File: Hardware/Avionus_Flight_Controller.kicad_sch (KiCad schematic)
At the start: 0 parts

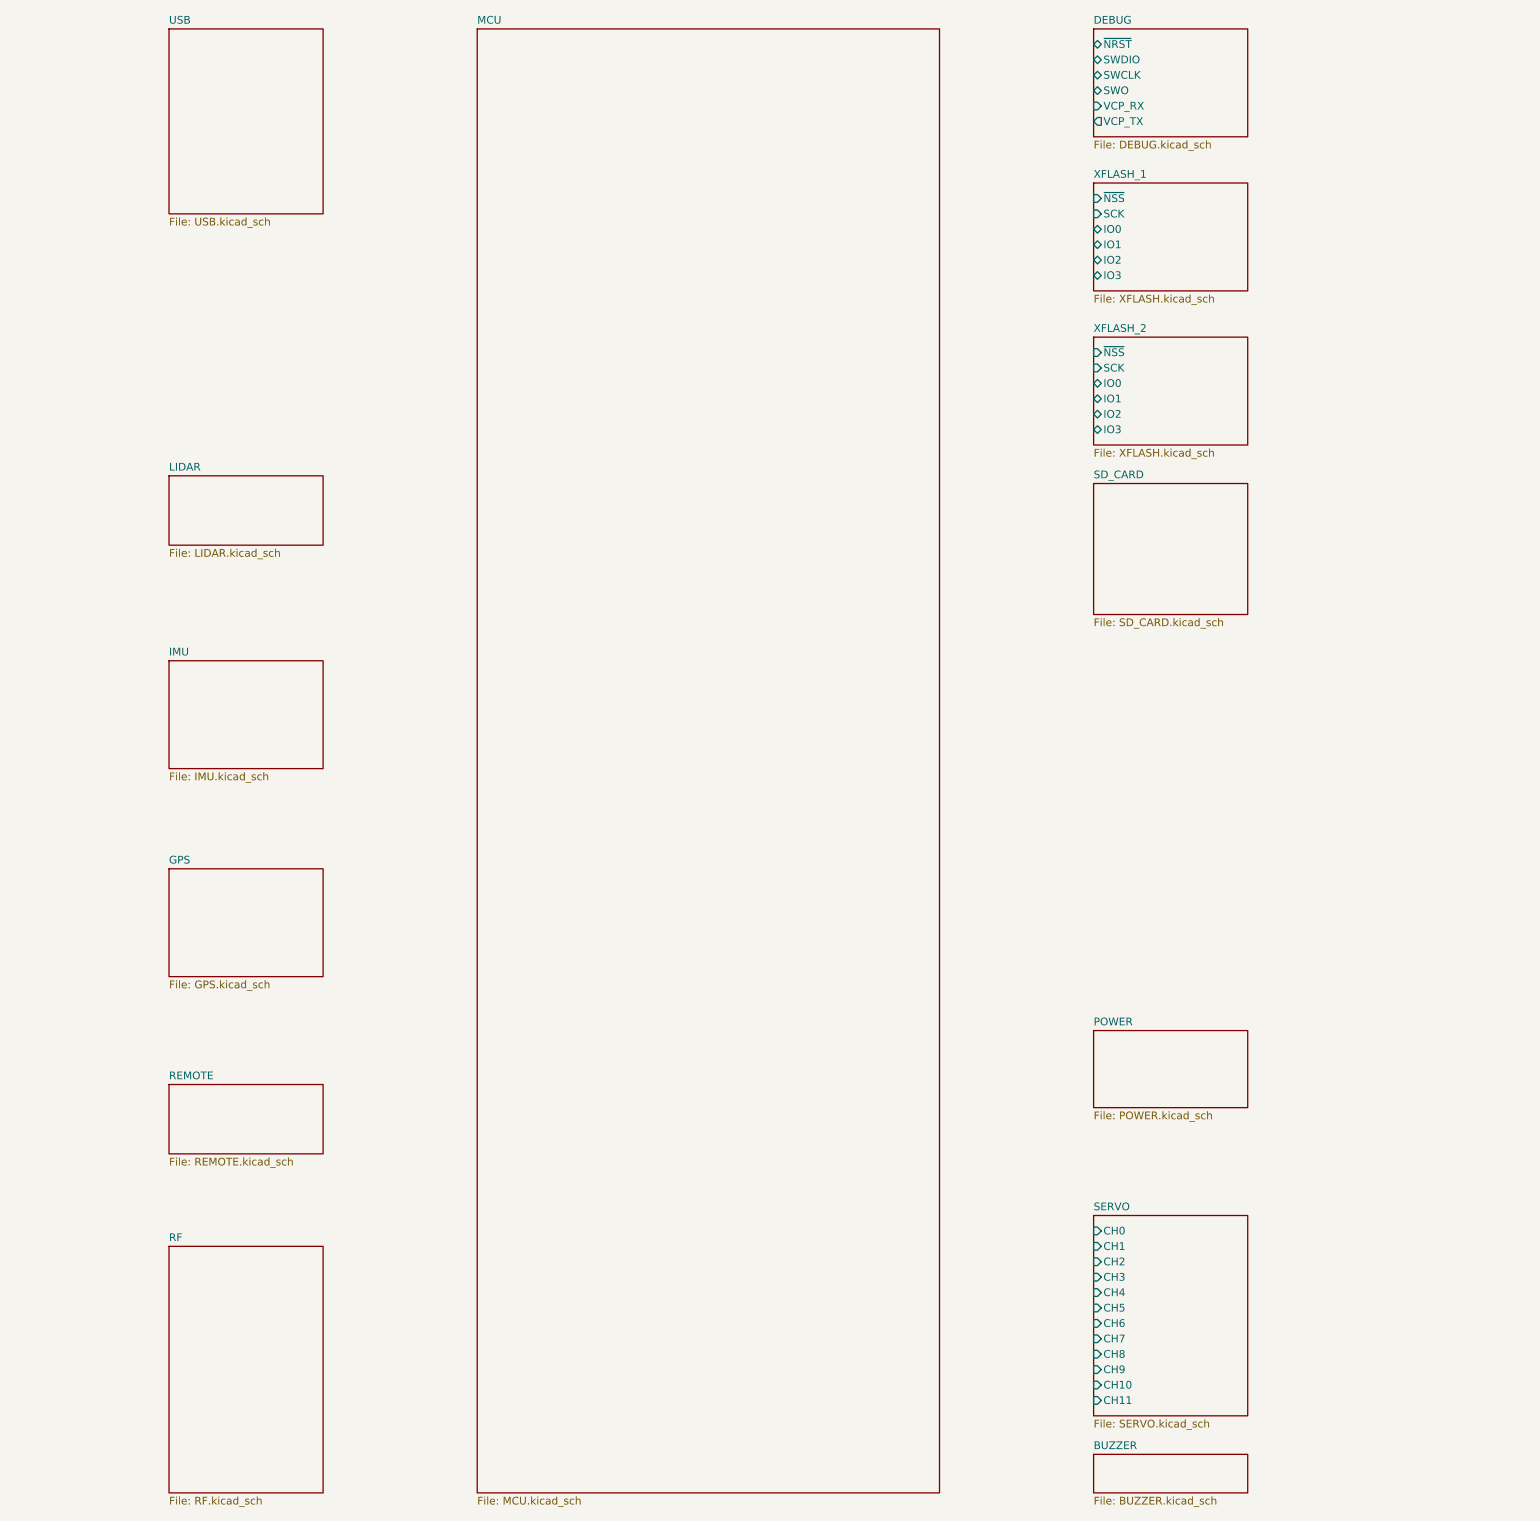
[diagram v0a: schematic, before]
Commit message: Checkpoint
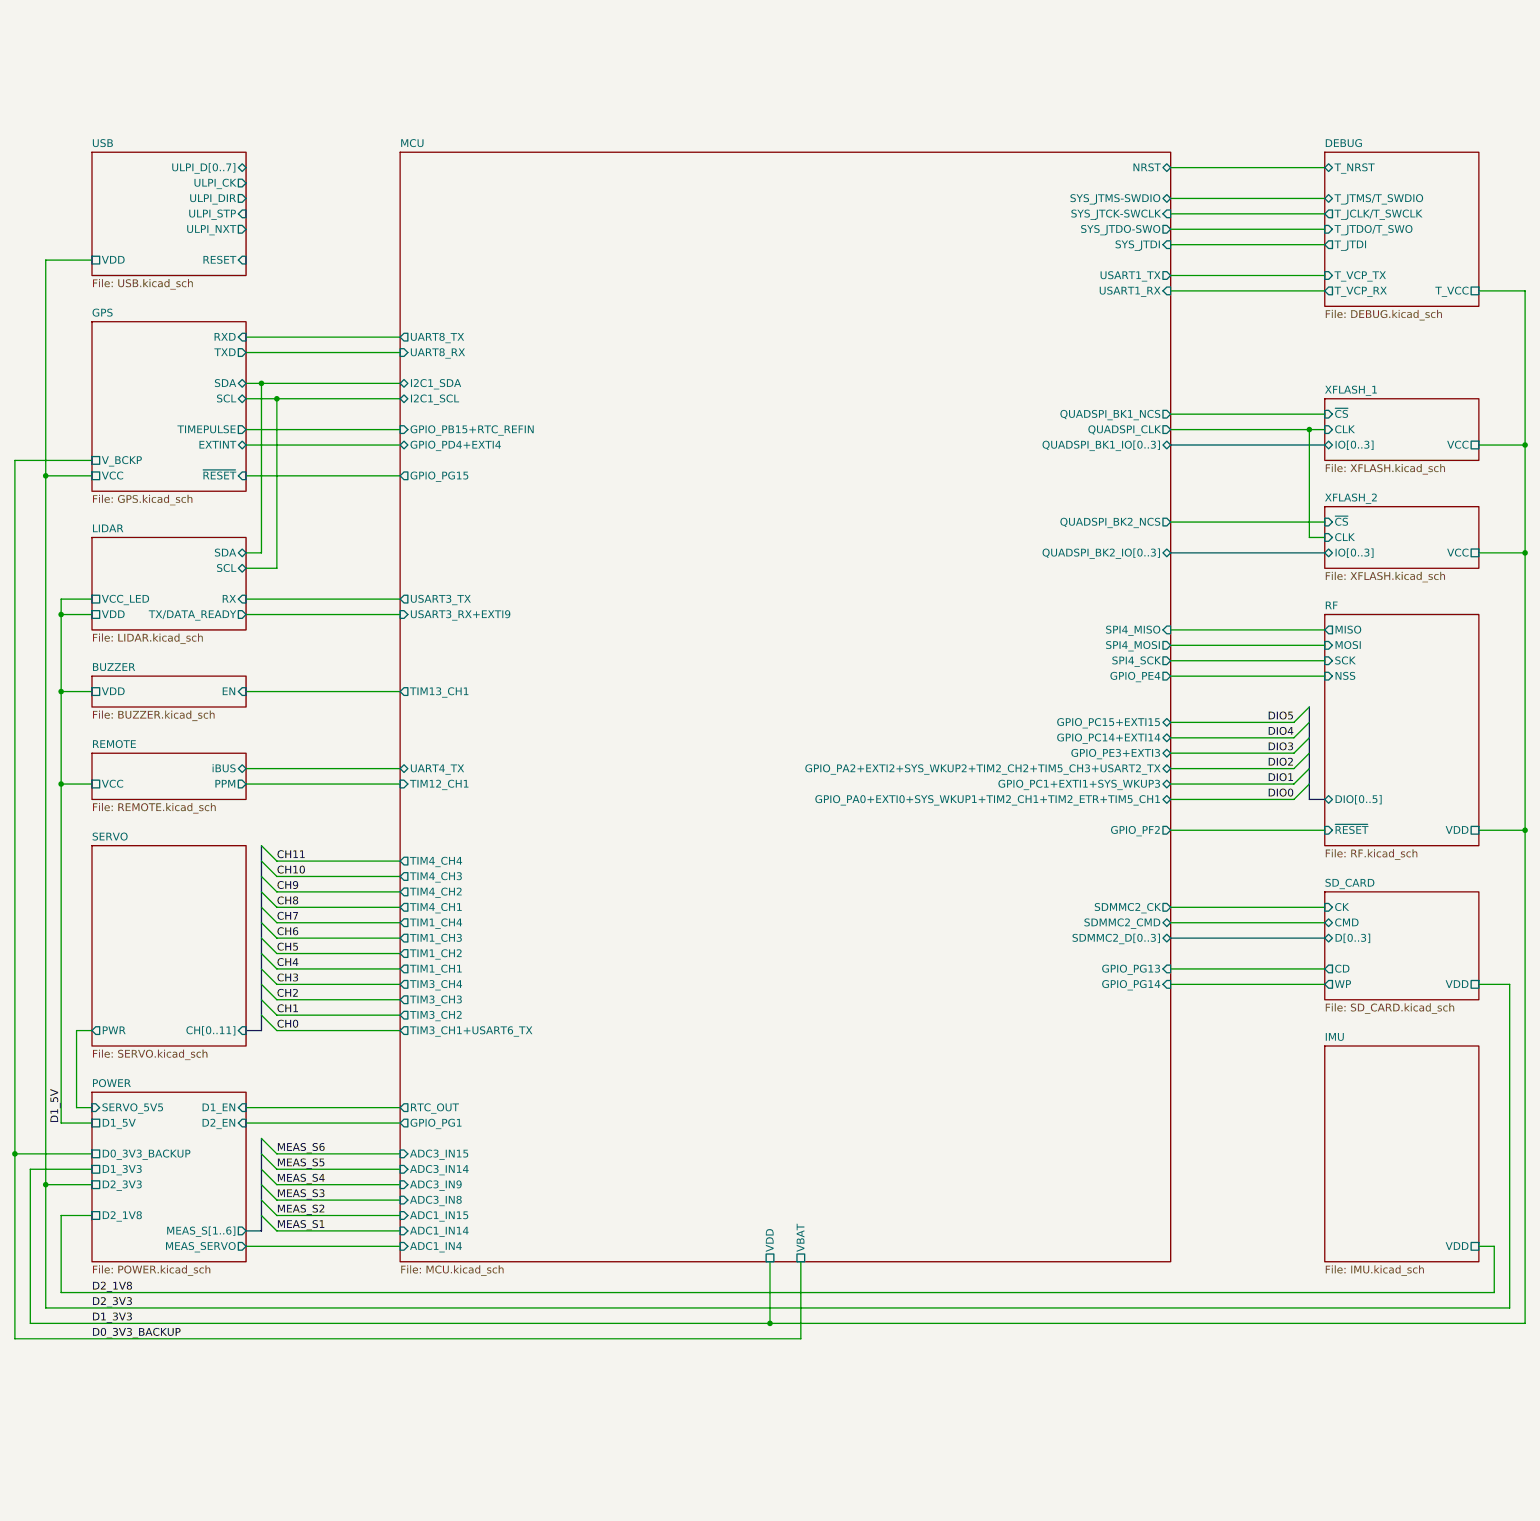
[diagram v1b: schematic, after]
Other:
- sheet BUZZER ports: added EN, VDD; removed none
- sheet DEBUG ports: added T_JCLK/T_SWCLK, T_JTDI, T_JTDO/T_SWO, T_JTMS/T_SWDIO, T_NRST , T_VCC, T_VCP_RX, T_VCP_TX; removed SWCLK, SWDIO, SWO, VCP_RX, VCP_TX, ~{NRST}
- sheet GPS ports: added EXTINT, RXD, SCL, SDA, TIMEPULSE, TXD, VCC, V_BCKP, ~{RESET}; removed none
- sheet IMU ports: added VDD; removed none
- sheet LIDAR ports: added RX, SCL, SDA, TX/DATA_READY, VCC_LED, VDD; removed none
- sheet MCU ports: added ADC1_IN14, ADC1_IN15, ADC1_IN4, ADC3_IN14, ADC3_IN15, ADC3_IN8, ADC3_IN9, GPIO_PA0+EXTI0+SYS_WKUP1+TIM2_CH1+TIM2_ETR+TIM5_CH1, GPIO_PA2+EXTI2+SYS_WKUP2+TIM2_CH2+TIM5_CH3+USART2_TX, GPIO_PB15+RTC_REFIN, GPIO_PC1+EXTI1+SYS_WKUP3, GPIO_PC14+EXTI14, GPIO_PC15+EXTI15, GPIO_PD4+EXTI4, GPIO_PE3+EXTI3, GPIO_PE4, GPIO_PF2, GPIO_PG1, GPIO_PG13, GPIO_PG14, GPIO_PG15, I2C1_SCL, I2C1_SDA, NRST, QUADSPI_BK1_IO[0..3], QUADSPI_BK1_NCS, QUADSPI_BK2_IO[0..3], QUADSPI_BK2_NCS, QUADSPI_CLK, RTC_OUT, SDMMC2_CK, SDMMC2_CMD, SDMMC2_D[0..3], SPI4_MISO, SPI4_MOSI, SPI4_SCK, SYS_JTCK-SWCLK, SYS_JTDI, SYS_JTDO-SWO, SYS_JTMS-SWDIO, TIM12_CH1, TIM13_CH1, TIM1_CH1, TIM1_CH2, TIM1_CH3, TIM1_CH4, TIM3_CH1+USART6_TX, TIM3_CH2, TIM3_CH3, TIM3_CH4, TIM4_CH1, TIM4_CH2, TIM4_CH3, TIM4_CH4, UART4_TX, UART8_RX, UART8_TX, USART1_RX, USART1_TX, USART3_RX+EXTI9, USART3_TX, VBAT, VDD; removed none
- sheet POWER ports: added D0_3V3_BACKUP, D1_3V3, D1_5V, D1_EN, D2_1V8, D2_3V3, D2_EN, MEAS_SERVO, MEAS_S[1..6], SERVO_5V5; removed none
- sheet REMOTE ports: added PPM, VCC, iBUS; removed none
- sheet RF ports: added DIO[0..5], MISO, MOSI, NSS, SCK, VDD, ~{RESET}; removed none
- sheet SD_CARD ports: added CD, CK, CMD, D[0..3], VDD, WP; removed none
- sheet SERVO ports: added CH[0..11], PWR; removed CH0, CH1, CH10, CH11, CH2, CH3, CH4, CH5, CH6, CH7, CH8, CH9
- sheet USB ports: added RESET, ULPI_CK, ULPI_DIR, ULPI_D[0..7], ULPI_NXT, ULPI_STP, VDD; removed none
- sheet XFLASH_1 ports: added CLK, IO[0..3], VCC, ~{CS}; removed IO0, IO1, IO2, IO3, SCK, ~{NSS}
- sheet XFLASH_2 ports: added CLK, IO[0..3], VCC, ~{CS}; removed IO0, IO1, IO2, IO3, SCK, ~{NSS}

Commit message: Checkpoint
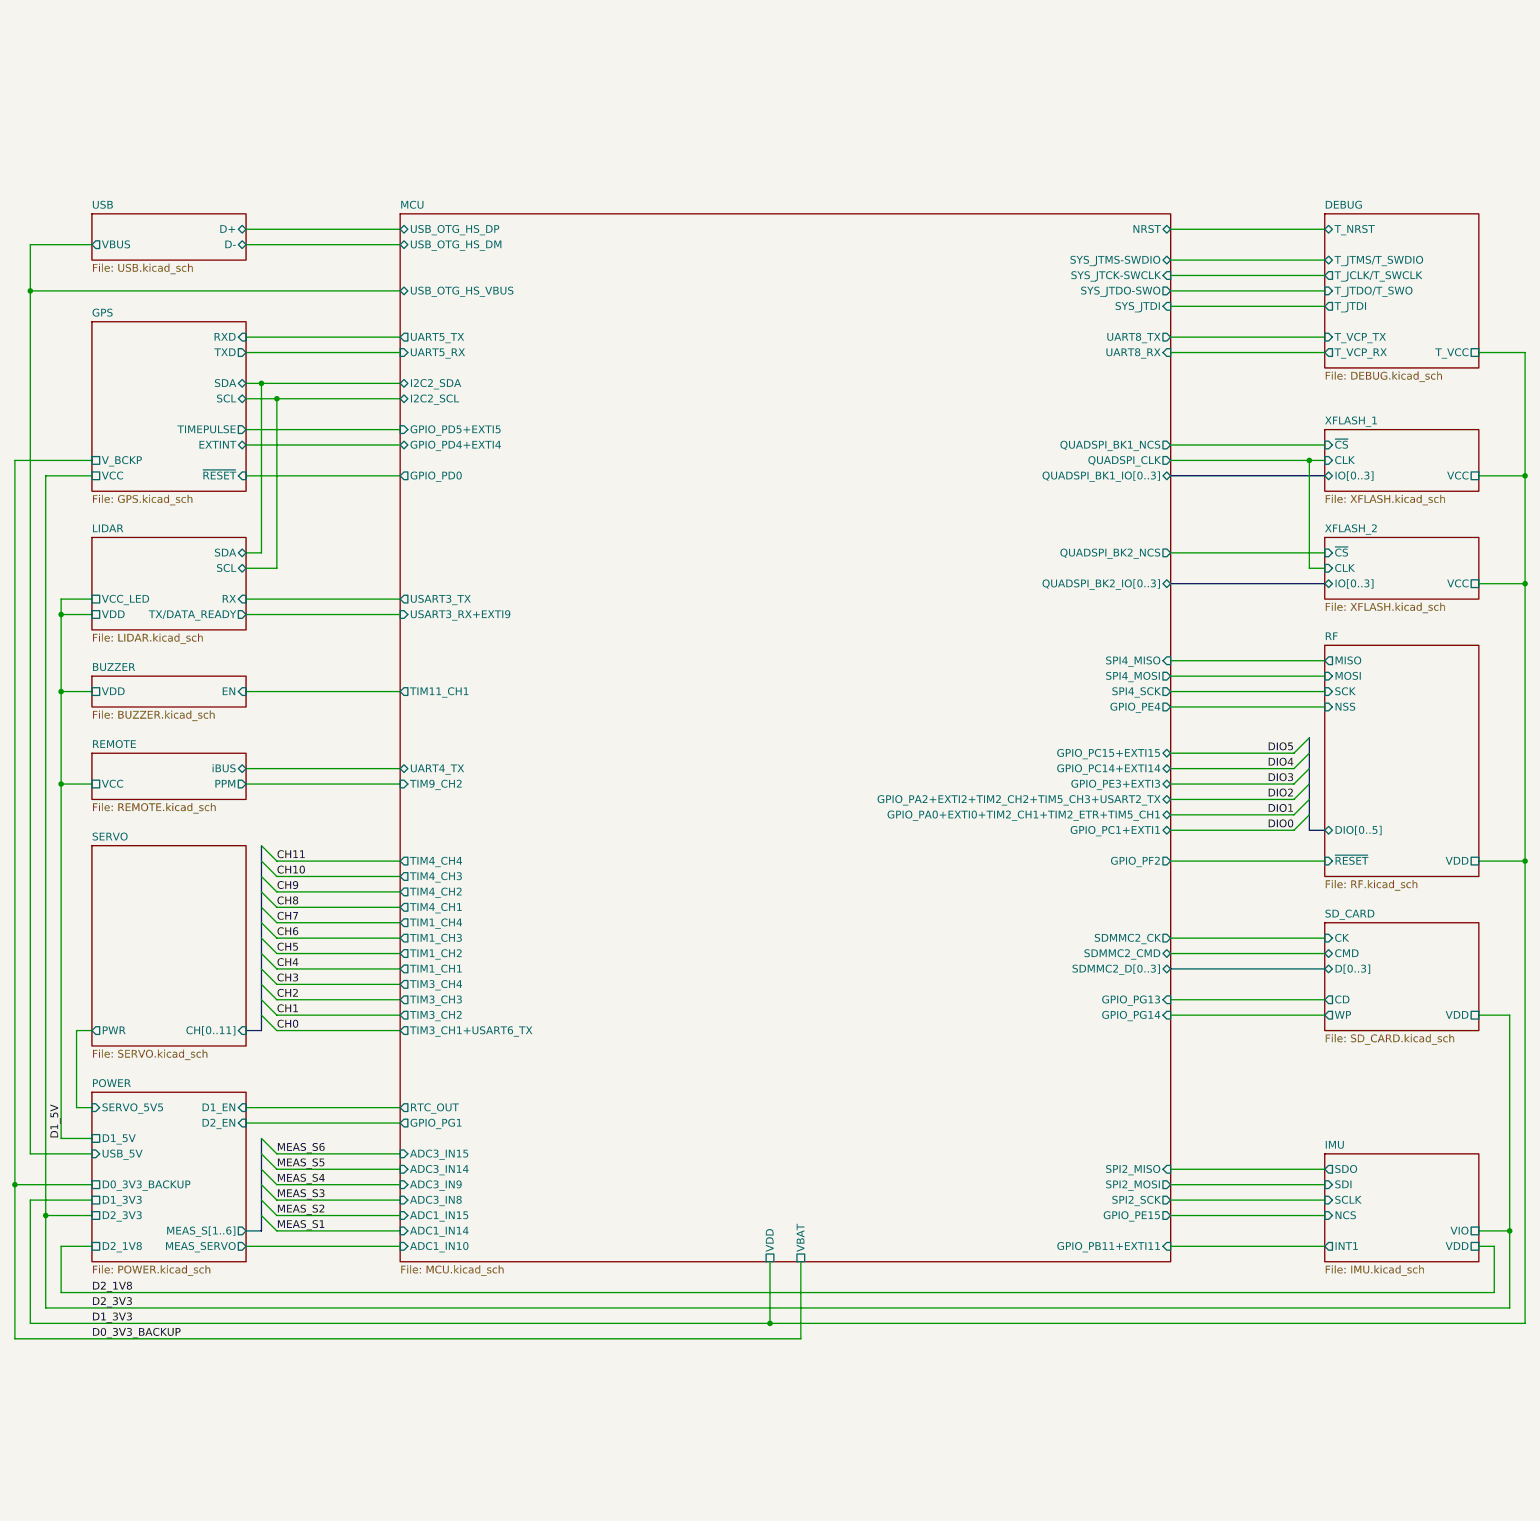
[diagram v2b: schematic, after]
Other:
- sheet IMU ports: added INT1, NCS, SCLK, SDI, SDO, VIO; removed none
- sheet MCU ports: added ADC1_IN10, GPIO_PA0+EXTI0+TIM2_CH1+TIM2_ETR+TIM5_CH1, GPIO_PA2+EXTI2+TIM2_CH2+TIM5_CH3+USART2_TX, GPIO_PB11+EXTI11, GPIO_PC1+EXTI1, GPIO_PD0, GPIO_PD5+EXTI5, GPIO_PE15, I2C2_SCL, I2C2_SDA, SPI2_MISO, SPI2_MOSI, SPI2_SCK, TIM11_CH1, TIM9_CH2, UART5_RX, UART5_TX, USB_OTG_HS_DM, USB_OTG_HS_DP, USB_OTG_HS_VBUS; removed ADC1_IN4, GPIO_PA0+EXTI0+SYS_WKUP1+TIM2_CH1+TIM2_ETR+TIM5_CH1, GPIO_PA2+EXTI2+SYS_WKUP2+TIM2_CH2+TIM5_CH3+USART2_TX, GPIO_PB15+RTC_REFIN, GPIO_PC1+EXTI1+SYS_WKUP3, GPIO_PG15, I2C1_SCL, I2C1_SDA, TIM12_CH1, TIM13_CH1, USART1_RX, USART1_TX
- sheet POWER ports: added USB_5V; removed none
- sheet USB ports: added D+, D-, VBUS; removed RESET, ULPI_CK, ULPI_DIR, ULPI_D[0..7], ULPI_NXT, ULPI_STP, VDD
